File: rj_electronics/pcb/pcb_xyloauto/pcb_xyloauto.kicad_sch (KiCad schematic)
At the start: 13 parts, among them J1 Conn_01x08_Pin, J2 Conn_01x08_Pin, J3 Conn_01x02_Pin, J4 Barrel_Jack, U1 Sparkfun_Pro_Micro, U2 ULN2803A, U3 LM317_TO-220

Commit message: nc
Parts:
- J4: footprint Connector Barrel Jack - Community:BarrelJack_GCT_DCJ200-10-A_Horizontal -> Connector Barrel Jack - Community:BarrelJack_Wuerth_6941xx301002
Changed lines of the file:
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@@
       (effects (font (size 1.27 1.27)))
     )
-    (property "Footprint" "Connector Barrel Jack - Community:BarrelJack_GCT_DCJ200-10-A_Horizontal" (at 116.84 31.496 0)
+    (property "Footprint" "Connector Barrel Jack - Community:BarrelJack_Wuerth_6941xx301002" (at 116.84 31.496 0)
       (effects (font (size 1.27 1.27)) hide)
     )

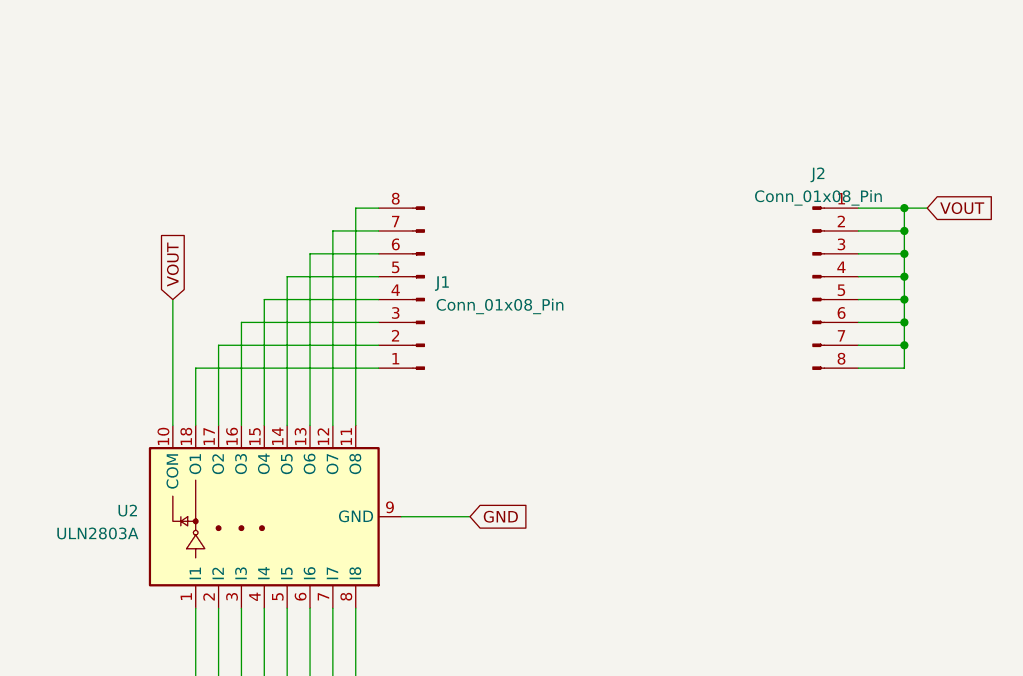
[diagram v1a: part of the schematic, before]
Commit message: nc
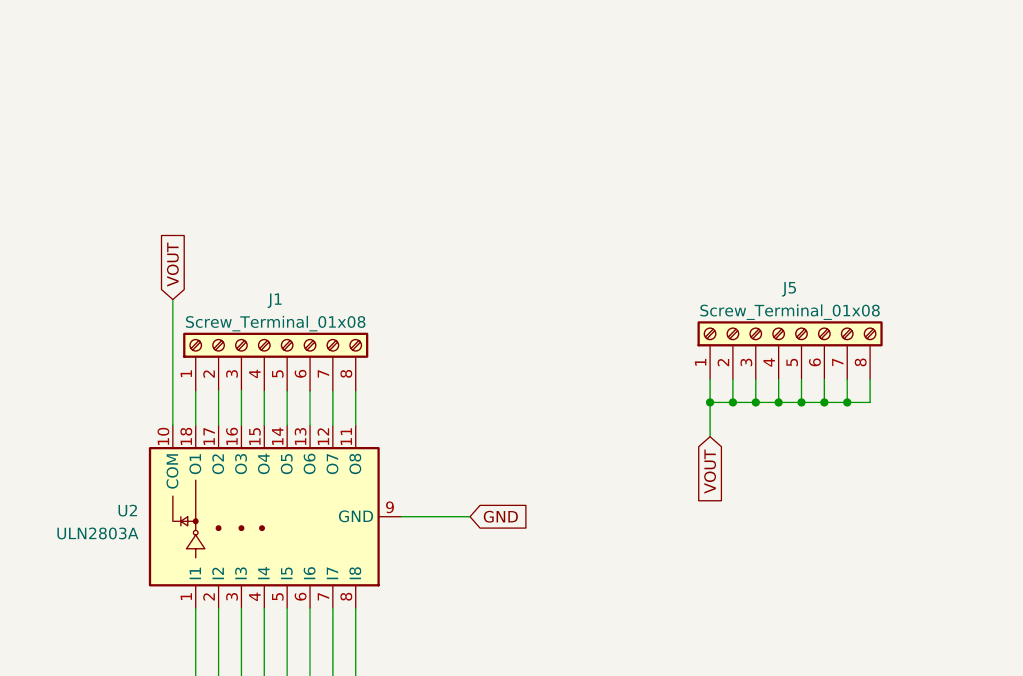
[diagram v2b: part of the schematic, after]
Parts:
- removed J1, J2: Conn_01x08_Pin, Connector_PinSocket_2.54mm:PinSocket_1x08_P2.54mm_Vertical, symbol Connector:Conn_01x08_Pin
- added J1, J5: Screw_Terminal_01x08, TerminalBlock_Phoenix:TerminalBlock_Phoenix_PT-1,5-8-3.5-H_1x08_P3.50mm_Horizontal, symbol Connector:Screw_Terminal_01x08
- R1: footprint Resistor_THT:R_Axial_DIN0414_L11.9mm_D4.5mm_P15.24mm_Horizontal -> Resistor_THT:R_Axial_DIN0207_L6.3mm_D2.5mm_P10.16mm_Horizontal
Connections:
- net VOUT: now also J5.1 (Pin_1), J5.2 (Pin_2), J5.3 (Pin_3), J5.4 (Pin_4), J5.5 (Pin_5), J5.6 (Pin_6), J5.7 (Pin_7), J5.8 (Pin_8)
- net at U2.11 (O8): now also J1.8 (Pin_8)
- net at U2.12 (O7): now also J1.7 (Pin_7)
- net at U2.13 (O6): now also J1.6 (Pin_6)
- net at U2.14 (O5): now also J1.5 (Pin_5)
- net at U2.15 (O4): now also J1.4 (Pin_4)
- net at U2.16 (O3): now also J1.3 (Pin_3)
- net at U2.17 (O2): now also J1.2 (Pin_2)
- net at U2.18 (O1): now also J1.1 (Pin_1)

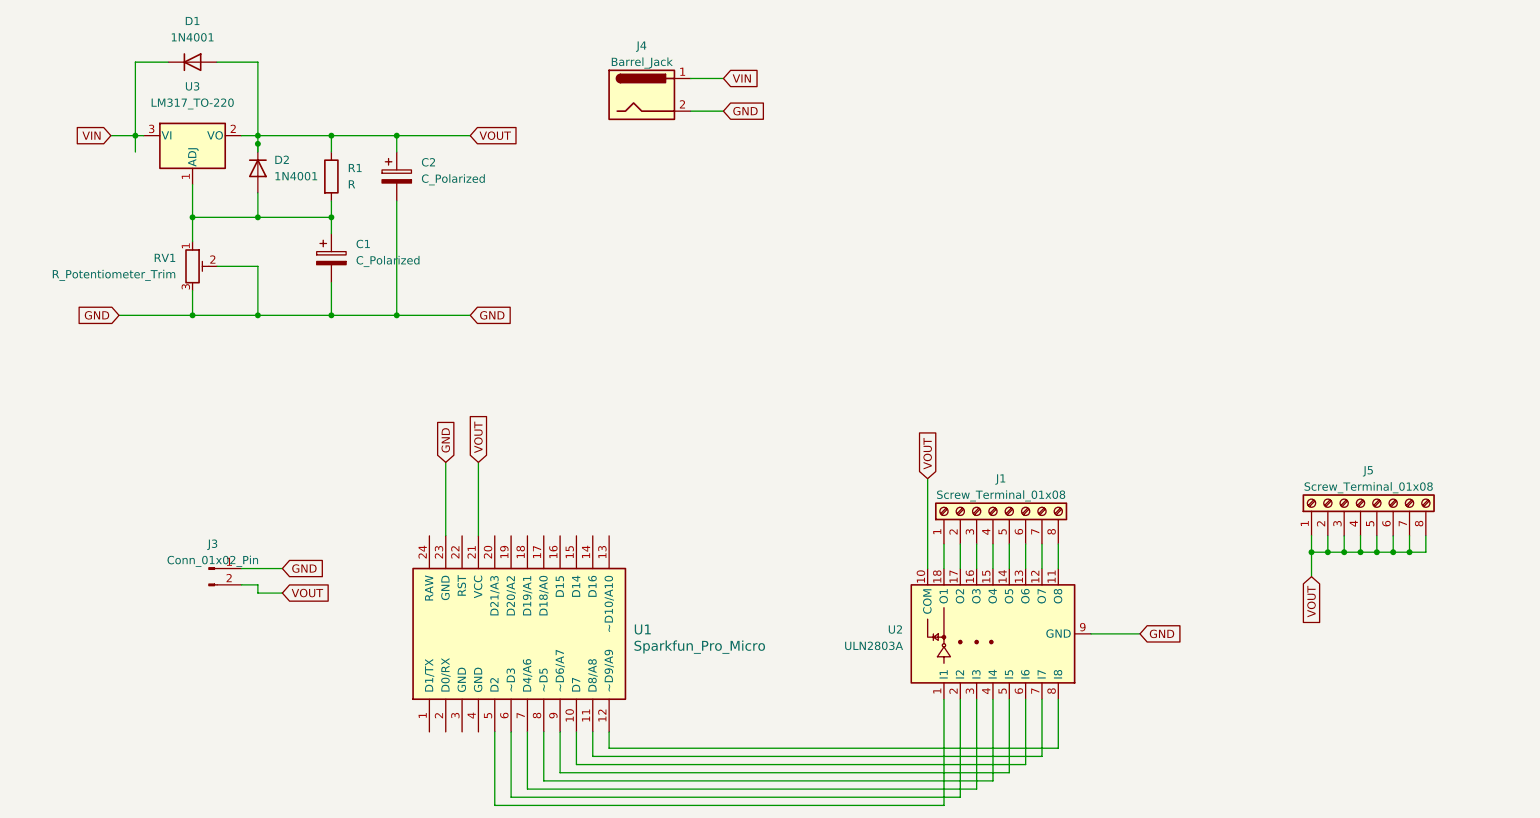
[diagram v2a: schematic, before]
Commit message: nc
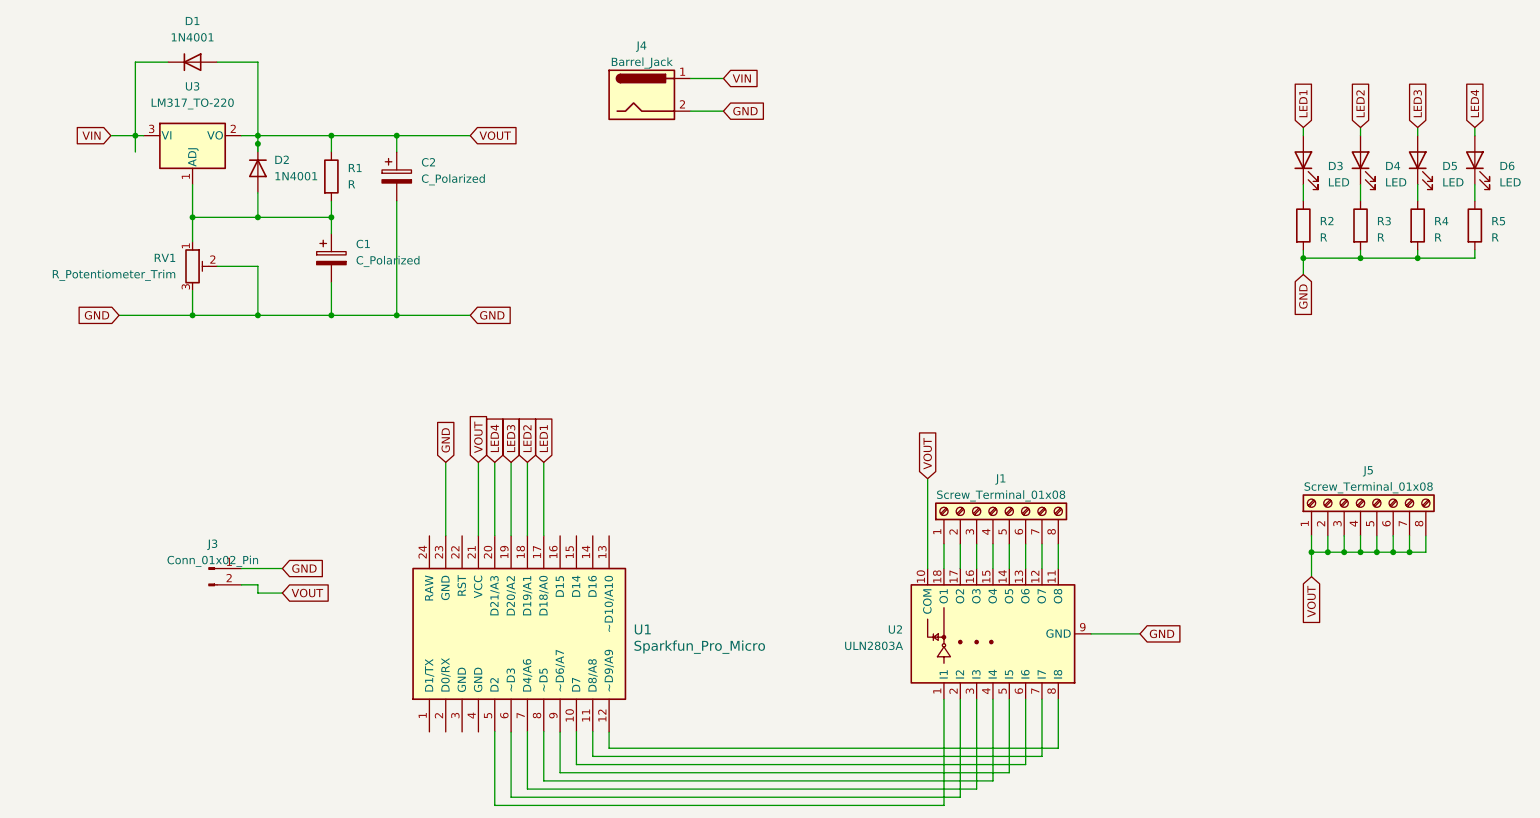
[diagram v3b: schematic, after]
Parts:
- added D3, D4, D5, D6: LED, LED_THT:LED_D5.0mm, symbol Device:LED
- added R2, R3, R4, R5: R, Resistor_THT:R_Axial_DIN0207_L6.3mm_D2.5mm_P10.16mm_Horizontal, symbol Device:R
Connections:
- net GND: now also R2.2, R3.2, R4.2, R5.2
- net LED1: now reaches U1.17 (D18/A0)
- net LED1: now also D3.2 (A)
- net LED2: now reaches U1.18 (D19/A1)
- net LED2: now also D4.2 (A)
- net LED3: now reaches U1.19 (D20/A2)
- net LED3: now also D5.2 (A)
- net LED4: now reaches U1.20 (D21/A3)
- net LED4: now also D6.2 (A)
- new net: D3.1 (K), R2.1
- new net: D5.1 (K), R4.1
- new net: D4.1 (K), R3.1
- new net: D6.1 (K), R5.1

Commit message: nc
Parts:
- RV1: footprint Potentiometer_THT:Potentiometer_Bourns_3339P_Vertical -> Potentiometer_THT:Potentiometer_Bourns_3299W_Vertical
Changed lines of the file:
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@@
       (effects (font (size 1.27 1.27)) (justify right))
     )
-    (property "Footprint" "Potentiometer_THT:Potentiometer_Bourns_3339P_Vertical" (at 45.72 57.15 0)
+    (property "Footprint" "Potentiometer_THT:Potentiometer_Bourns_3299W_Vertical" (at 45.72 57.15 0)
       (effects (font (size 1.27 1.27)) hide)
     )
